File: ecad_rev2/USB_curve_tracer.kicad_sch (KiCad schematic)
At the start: 60 parts, among them J2 Programmer Header, J3 USB_A, U2 MCP2221AxSL

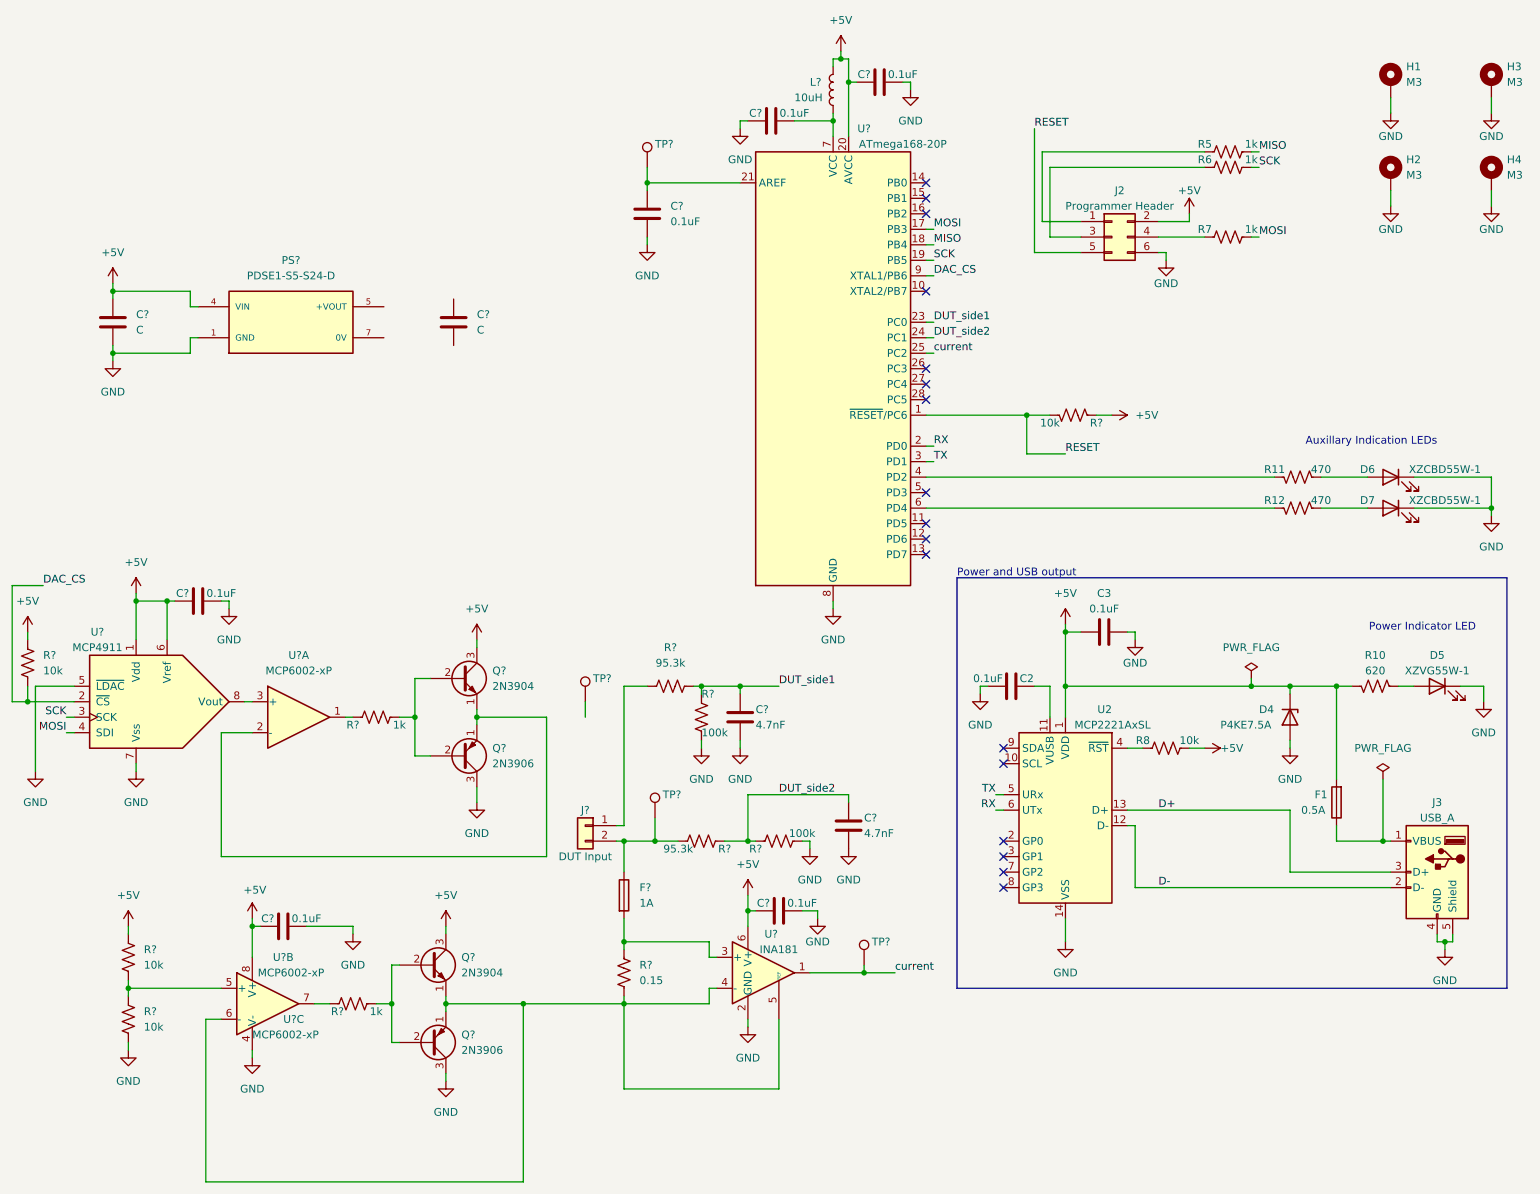
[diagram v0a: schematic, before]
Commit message: solid front end
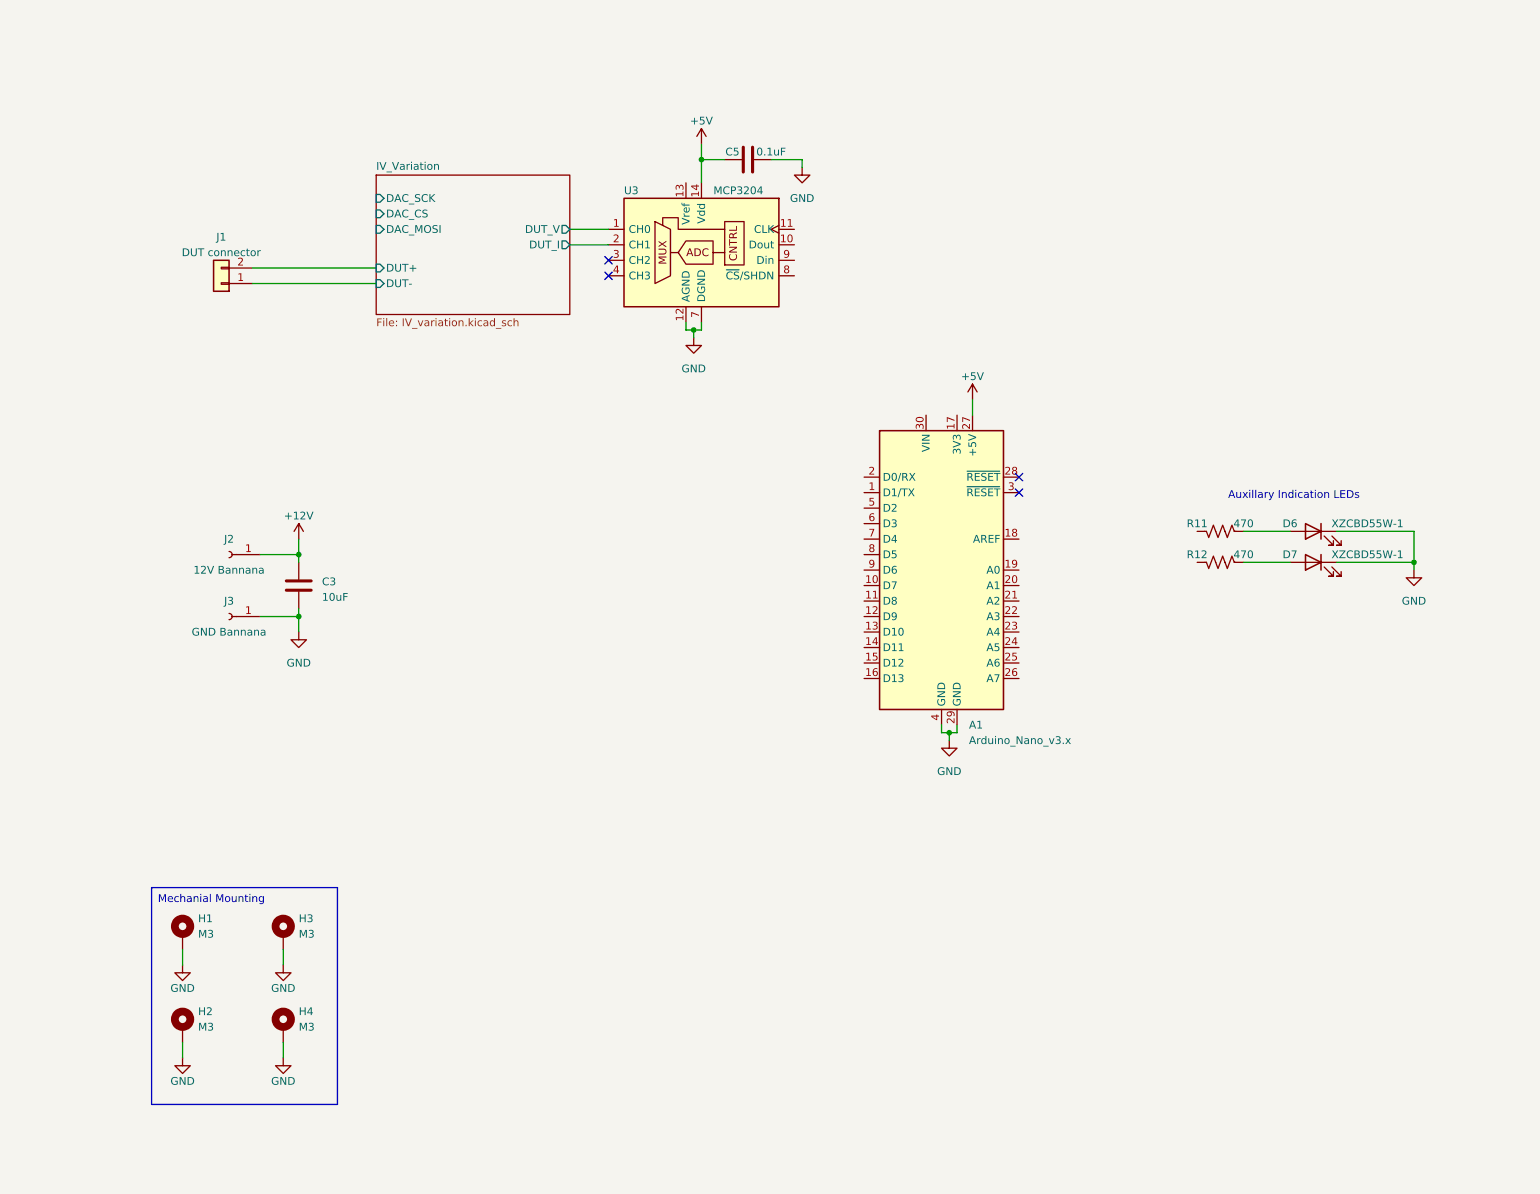
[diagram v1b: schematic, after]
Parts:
- removed C2: 0.1uF, Capacitor_THT:C_Disc_D6.0mm_W2.5mm_P5.00mm, symbol Device:C
- removed C? (x2): C, symbol Device:C
- removed C? (x6): 0.1uF, symbol Device:C
- removed C? (x2): 4.7nF, symbol Device:C
- removed D4: P4KE7.5A, Diode_THT:D_DO-41_SOD81_P7.62mm_Horizontal, symbol Device:D_Zener
- removed D5: XZVG55W-1, LED_SMD:LED_1206_3216Metric_Pad1.42x1.75mm_HandSolder, symbol Device:LED
- removed F1: 0.5A, Fuse:Fuse_1206_3216Metric_Pad1.42x1.75mm_HandSolder, symbol Device:Fuse
- removed F?: 1A, symbol Device:Fuse
- removed J2: Programmer Header, Connector_PinSocket_2.54mm:PinSocket_2x03_P2.54mm_Vertical, symbol Connector_Generic:Conn_02x03_Odd_Even
- removed J3: USB_A, Connector_USB:USB_B_OST_USB-B1HSxx_Horizontal, symbol Connector:USB_A
- removed J?: DUT Input, symbol Connector_Generic:Conn_01x02
- removed L?: 10uH, symbol Device:L
- removed PS?: PDSE1-S5-S24-D, symbol USB_curve_tracer_parts:PDSE1-S5-S24-D
- removed Q? (x2): 2N3906, Package_TO_SOT_THT:TO-92_Inline, symbol Transistor_BJT:2N3906
- removed Q? (x2): 2N3904, Package_TO_SOT_THT:TO-92_Inline, symbol Transistor_BJT:2N3904
- removed R10: 620, Resistor_THT:R_Axial_DIN0207_L6.3mm_D2.5mm_P7.62mm_Horizontal, symbol Device:R_US
- removed R5, R6, R7: 1k, Resistor_THT:R_Axial_DIN0207_L6.3mm_D2.5mm_P7.62mm_Horizontal, symbol Device:R_US
- removed R8: 10k, Resistor_THT:R_Axial_DIN0207_L6.3mm_D2.5mm_P7.62mm_Horizontal, symbol Device:R_US
- removed R? (x4): 10k, symbol Device:R_US
- removed R? (x2): 1k, symbol Device:R_US
- removed R? (x2): 95.3k, symbol Device:R_US
- removed R? (x2): 100k, symbol Device:R_US
- removed R?: 0.15, symbol Device:R_US
- removed TP? (x4): ~, symbol Connector:TestPoint
- removed U2: MCP2221AxSL, Package_SO:SOIC-14_3.9x8.7mm_P1.27mm, symbol Interface_USB:MCP2221AxSL
- removed U? (x3): MCP6002-xP, symbol Amplifier_Operational:MCP6002-xP
- removed U?: ATmega168-20P, Package_DIP:DIP-28_W7.62mm, symbol MCU_Microchip_ATmega:ATmega168-20P
- removed U?: MCP4911, symbol Analog_DAC:MCP4911
- removed U?: INA181, Package_TO_SOT_SMD:SOT-23-6, symbol Amplifier_Current:INA181
- added A1: Arduino_Nano_v3.x, Module:Arduino_Nano, symbol MCU_Module:Arduino_Nano_v3.x
- added C5: 0.1uF, symbol Device:C
- added J1: DUT connector, symbol Connector_Generic:Conn_01x02
- added J2: 12V Bannana, symbol Connector:Conn_01x01_Socket
- added J3: GND Bannana, symbol Connector:Conn_01x01_Socket
- added U3: MCP3204, symbol Analog_ADC:MCP3204
- C3: value 0.1uF -> 10uF; footprint Capacitor_THT:C_Disc_D6.0mm_W2.5mm_P5.00mm -> (none)
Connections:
- net +5V: now also A1.27 (+5V), C5.1, U3.14 (Vdd); no longer C3.2
- net GND: now also C3.2, A1.29 (GND), A1.4 (GND), C5.2, J3.1 (Pin_1), U3.12 (AGND), U3.7 (DGND); no longer C3.1
- new net +12V: C3.1, J2.1 (Pin_1)
- new net IV_Variation/DUT+: J1.2 (Pin_2)
- new net IV_Variation/DUT-: J1.1 (Pin_1)
- new net IV_Variation/DUT_I: U3.2 (CH1)
- new net IV_Variation/DUT_V: U3.1 (CH0)
- no-connect marks 17 -> 4
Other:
- added sheet IV_Variation (IV_variation.kicad_sch)
- note removed: "Power Indicator LED"
- note removed: "Power and USB output"
- moved on the sheet: D6, D7, H1, H2, H3, H4, R11, R12

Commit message: schematic work
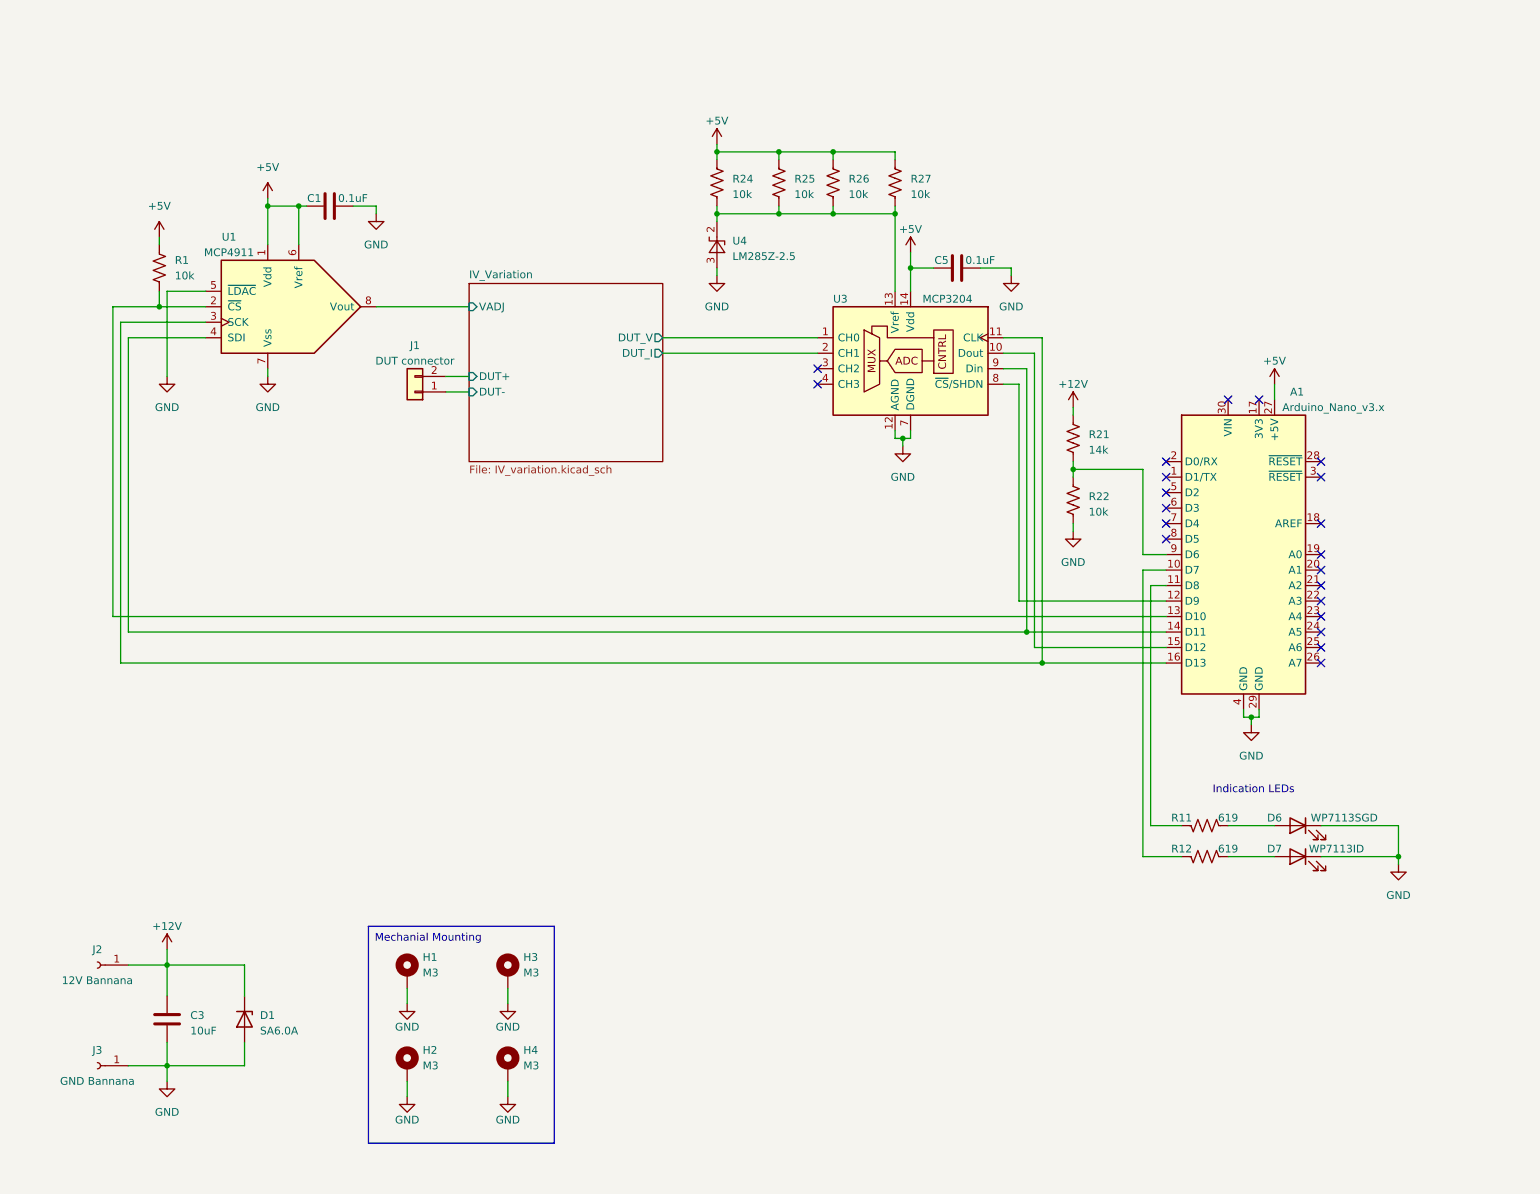
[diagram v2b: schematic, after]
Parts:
- added C1: 0.1uF, Capacitor_THT:C_Disc_D6.0mm_W2.5mm_P5.00mm, symbol Device:C
- added D1: SA6.0A, symbol Device:D_Zener
- added R1, R22, R24, R25, R26, R27: 10k, Resistor_THT:R_Axial_DIN0207_L6.3mm_D2.5mm_P7.62mm_Horizontal, symbol Device:R_US
- added R21: 14k, Resistor_THT:R_Axial_DIN0207_L6.3mm_D2.5mm_P7.62mm_Horizontal, symbol Device:R_US
- added U1: MCP4911, symbol Analog_DAC:MCP4911
- added U4: LM285Z-2.5, Package_TO_SOT_THT:TO-92_Inline, symbol Reference_Voltage:LM285Z-2.5
- C3, C5: footprint (none) -> Capacitor_THT:C_Disc_D6.0mm_W2.5mm_P5.00mm
- D6: value XZCBD55W-1 -> WP7113SGD
- D7: value XZCBD55W-1 -> WP7113ID
- H1, H2, H3, H4: now left out of the parts list
- R11, R12: value 470 -> 619
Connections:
- net +12V: now also D1.1 (K), R21.1
- net +5V: now also C1.1, R1.1, R24.1, R25.1, R26.1, R27.1, U1.1 (Vdd), U1.6 (Vref)
- net GND: now also C1.2, D1.2 (A), R22.2, U1.5 (~{LDAC}), U1.7 (Vss), U4.3 (A)
- net at R11.2: now also A1.11 (D8)
- net at U3.10 (Dout): now also A1.15 (D12)
- net at U3.11 (CLK): now also A1.16 (D13), U1.3 (SCK)
- net at U3.13 (Vref): now also R24.2, R25.2, R26.2, R27.2, U4.2 (K)
- net at U3.8 (~{CS}/SHDN): now also A1.12 (D9)
- net at U3.9 (Din): now also A1.14 (D11), U1.4 (SDI)
- net at R12.2: now also A1.10 (D7)
- net at A1.13 (D10): now also R1.2, U1.2 (~{CS})
- net at A1.9 (D6): now also R21.2, R22.1
- new net IV_Variation/VADJ: U1.8 (Vout)
- no-connect marks 4 -> 21
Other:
- sheet IV_Variation ports: added VADJ; removed DAC_CS, DAC_MOSI, DAC_SCK
- note added: "Indication LEDs"
- note removed: "Auxillary Indication LEDs"
- moved on the sheet: A1, C3, C5, D6, D7, H1, H2, H3, H4, J1, J2, J3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
